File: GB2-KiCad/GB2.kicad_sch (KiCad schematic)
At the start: 43 parts, among them J1 Screw_Terminal_01x02, J2 Screw_Terminal_01x02, J3 Barrel_Jack_Switch, J4 Conn_02x10_Odd_Even, T1 Transformer_1P_2S, U7 L7805, U8 L7812/L7815

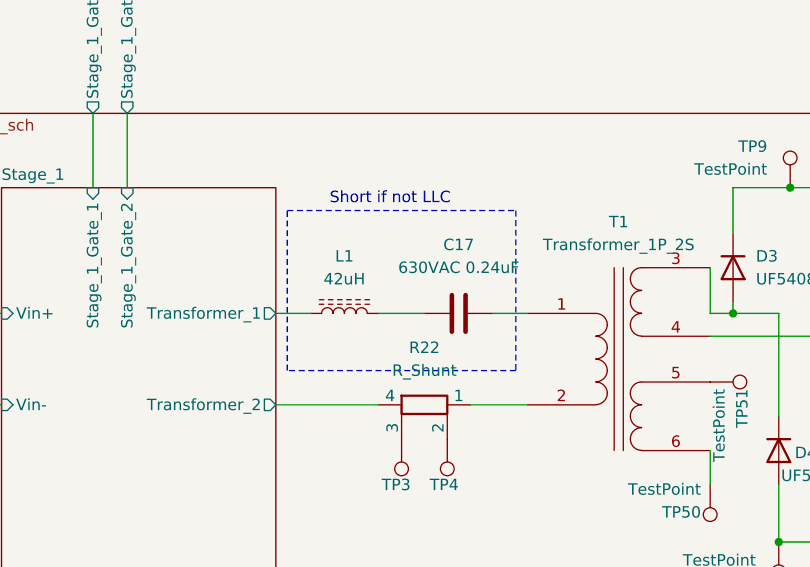
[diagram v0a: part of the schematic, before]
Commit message: Full pcb layout update
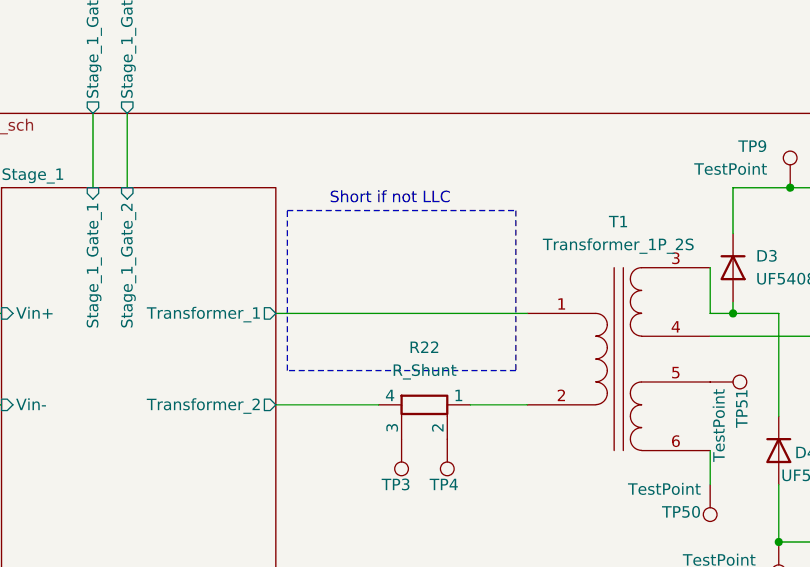
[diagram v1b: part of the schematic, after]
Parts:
- removed C17: 630VAC 0.24uF, Capacitor_THT:C_Rect_L33.0mm_W15.0mm_P27.50mm_MKS4, symbol Device:C
- removed L1: 42uH, Inductor_THT:L_Toroid_Vertical_L21.6mm_W8.4mm_P8.38mm_Pulse_G, symbol Device:L_Ferrite
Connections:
- net Stage_1/Transformer_1: now also T1.1 (AA)
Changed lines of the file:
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@@
-	(wire
-		(pts
-			(xy 109.22 115.57) (xy 114.3 115.57)
-		)
-		(stroke
-			(width 0)
-			(type default)
-		)
-	)
 	(wire
 		(pts
@@
 	(wire
 		(pts
-			(xy 97.79 115.57) (xy 101.6 115.57)
-		)
-		(stroke
-			(width 0)
-			(type default)
-		)
-	)
-	(wire
-		(pts
-			(xy 121.92 115.57) (xy 125.73 115.57)
+			(xy 97.79 115.57) (xy 125.73 115.57)
 		)
 		(stroke
@@
 	)
 	(symbol
-		(lib_id "Device:L_Ferrite")
-		(at 105.41 115.57 90)
-		(unit 1)
-		(exclude_from_sim no)
-		(in_bom yes)
-		(on_board yes)
-		(dnp no)
-		(fields_autoplaced yes)
-		(property "Reference" "L1"
-			(at 105.41 109.22 90)
-			(effects
-				(font
-					(size 1.27 1.27)
-				)
-			)
-		)
-		(property "Value" "42uH"
-			(at 105.41 111.76 90)
-			(effects
-				(font
-					(size 1.27 1.27)
-				)
-			)
-		)
-		(property "Footprint" "Inductor_THT:L_Toroid_Vertical_L21.6mm_W8.4mm_P8.38mm_Pulse_G"
-			(at 105.41 115.57 0)
-			(effects
-				(font
-					(size 1.27 1.27)
-				)
-				(hide yes)
-			)
-		)
-		(property "Datasheet" "~"
-			(at 105.41 115.57 0)
-			(effects
-				(font
-					(size 1.27 1.27)
-				)
-				(hide yes)
-			)
-		)
-		(property "Description" "Inductor with ferrite core"
-			(at 105.41 115.57 0)
-			(effects
-				(font
-					(size 1.27 1.27)
-				)
-				(hide yes)
-			)
-		)
-		(pin "1"
-		)
-		(pin "2"
-		)
-		(instances
-			(project ""
-				(path "/bf64a716-2fc8-4393-9642-a6408cd72f3a"
-					(reference "L1")
-					(unit 1)
-				)
-			)
-		)
-	)
-	(symbol
 		(lib_id "Device:C_Polarized")
 		(at 46.99 120.65 0)
@@
 					(unit 1)
 				)
-			)
-		)
-	)
-	(symbol
-		(lib_id "Device:C")
-		(at 118.11 115.57 90)
-		(unit 1)
-		(exclude_from_sim no)
-		(in_bom yes)
-		(on_board yes)
-		(dnp no)
-		(fields_autoplaced yes)
-		(property "Reference" "C17"
-			(at 118.11 107.95 90)
-			(effects
-				(font
-					(size 1.27 1.27)
-				)
-			)
-		)
-		(property "Value" "630VAC 0.24uF"
-			(at 118.11 110.49 90)
-			(effects
-				(font
-					(size 1.27 1.27)
-				)
-			)
-		)
-		(property "Footprint" "Capacitor_THT:C_Rect_L33.0mm_W15.0mm_P27.50mm_MKS4"
-			(at 121.92 114.6048 0)
-			(effects
-				(font
-					(size 1.27 1.27)
-				)
-				(hide yes)
-			)
-		)
-		(property "Datasheet" "~"
-			(at 118.11 115.57 0)
-			(effects
-				(font
-					(size 1.27 1.27)
-				)
-				(hide yes)
-			)
-		)
-		(property "Description" "Unpolarized capacitor"
-			(at 118.11 115.57 0)
-			(effects
-				(font
-					(size 1.27 1.27)
-				)
-				(hide yes)
-			)
-		)
-		(pin "2"
-		)
-		(pin "1"
-		)
-		(instances
-			(project ""
-				(path "/bf64a716-2fc8-4393-9642-a6408cd72f3a"
-					(reference "C17")
-					(unit 1)
-				)
